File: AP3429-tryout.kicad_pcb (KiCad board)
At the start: 2 copper layers, 90 x 50 mm, 61 parts, among them J1 Conn_01x05, J2 Conn_01x02, U1 AP3429, U10 AMS1117-3.3, U2 AP3429, U3 AP3429, U4 AP2120N, U5 AMS1117-3.3, U6 AMS1117-3.3, U7 AMS1117-3.3, U8 AMS1117-3.3, U9 AMS1117-3.3

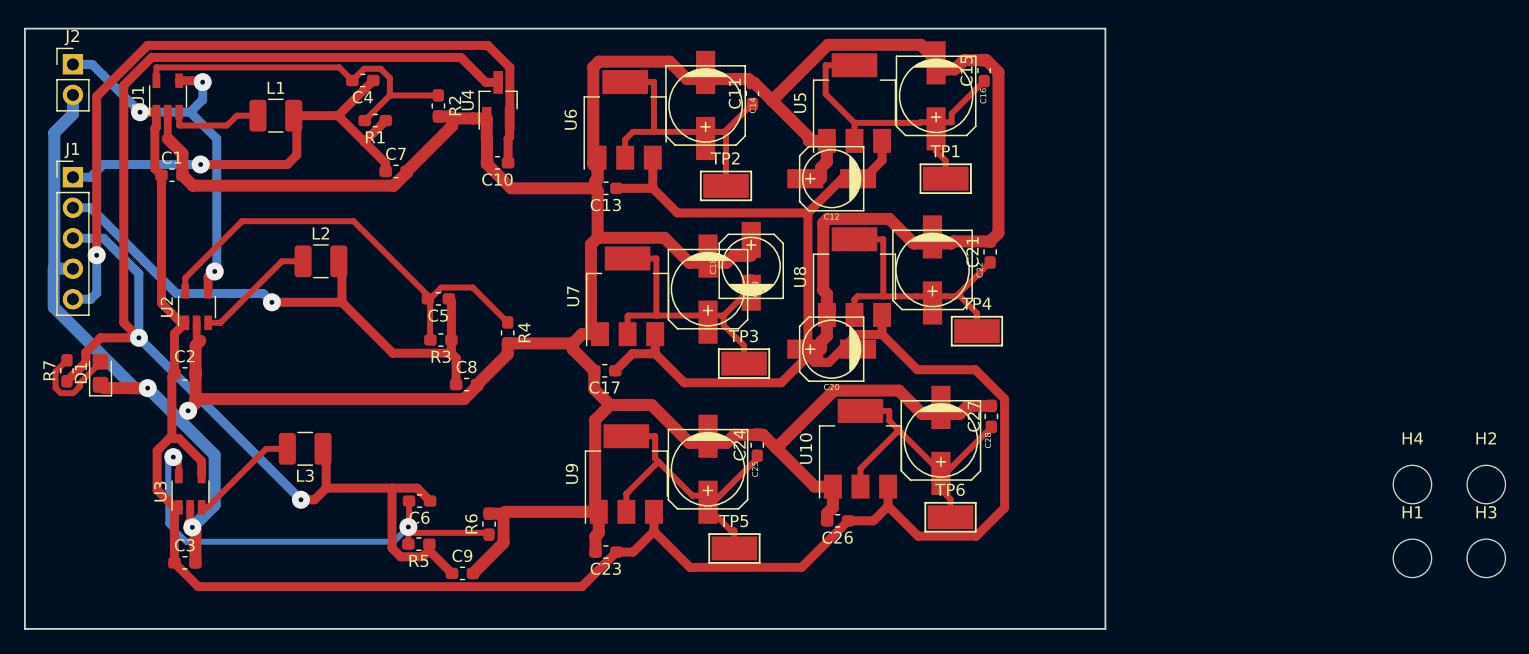
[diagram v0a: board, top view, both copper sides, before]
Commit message: update,
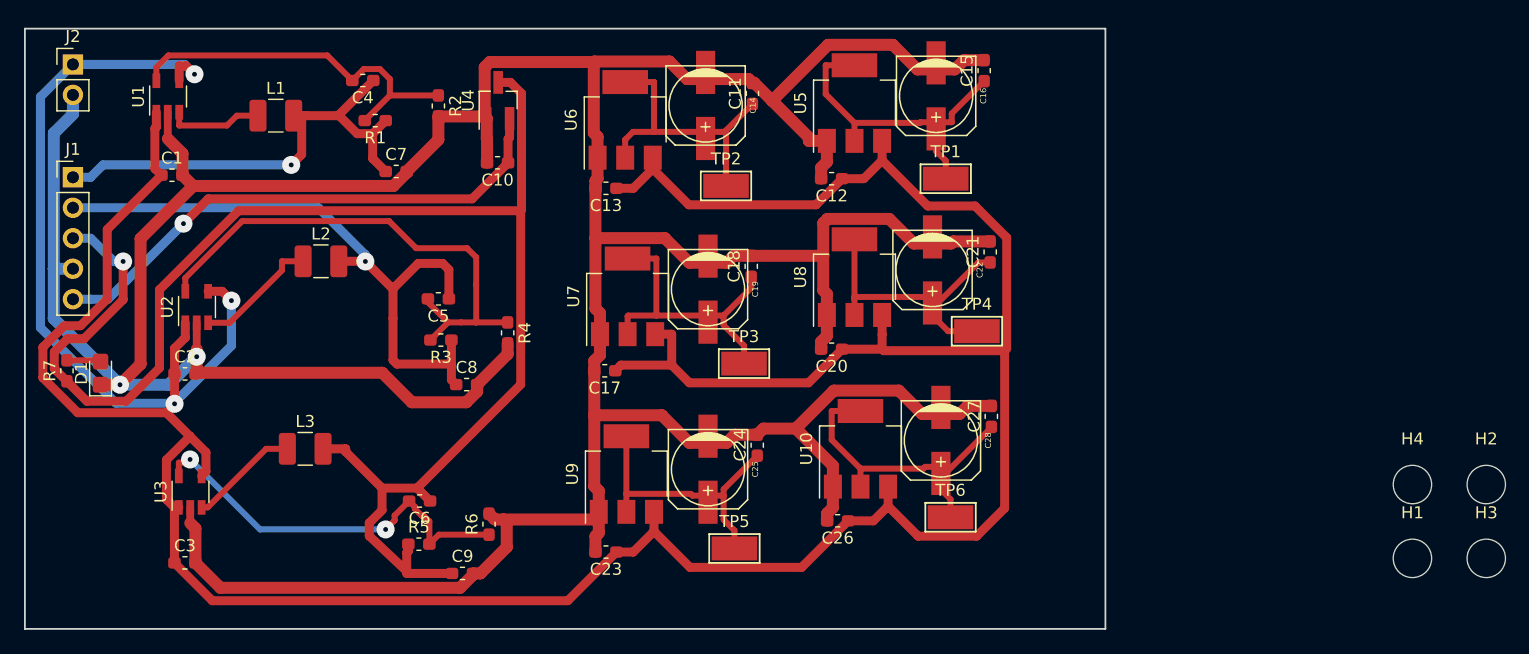
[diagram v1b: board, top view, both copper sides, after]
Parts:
- C12, C18, C20: footprint w_smd_cap:c_elec_5x5.3 -> Capacitor_SMD:C_0603_1608Metric_Pad1.05x0.95mm_HandSolder
- turned L3 to 0 degrees
- turned R5 to 0 degrees
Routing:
- net +5V: track 251.3 -> 315.1 mm
- net +3V0: track 64.3 -> 44.7 mm
- net GND: track 355.9 -> 367.9 mm, vias 3 -> 2
- net +3V3: track 120.4 -> 131.8 mm, vias 2 -> 1
- net +1V8: track 47.3 -> 54.7 mm
- net Net-(C5-Pad2): track 37.8 -> 43.7 mm
- net Net-(C6-Pad2): track 39.0 -> 33.7 mm
- net Net-(D1-Pad2): track 7.91 -> 2.85 mm
- net Net-(C24-Pad1): track 26.7 -> 23.7 mm
- net Net-(C27-Pad1): track 25.9 -> 27.0 mm
- net Net-(C4-Pad2): track 30.2 -> 30.9 mm
- net Net-(C21-Pad1): track 24.7 -> 25.4 mm
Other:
- net class Default: clearance 0.2 -> 0.5
- net class GND: clearance 0.2 -> 0.5
- net class PWR: clearance 0.2 -> 0.5
- rule trace_clearance: 0.2 -> 0.5
